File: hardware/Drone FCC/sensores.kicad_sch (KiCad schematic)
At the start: 17 parts, among them J1 Conn_02x03_Counter_Clockwise, J19 GPS M8N, J2 Conector GPS Auxiliar, J20 Conector Magnetómetro I2C DF13, U1 ICM-42688-V, U2 ILPS22QSTR

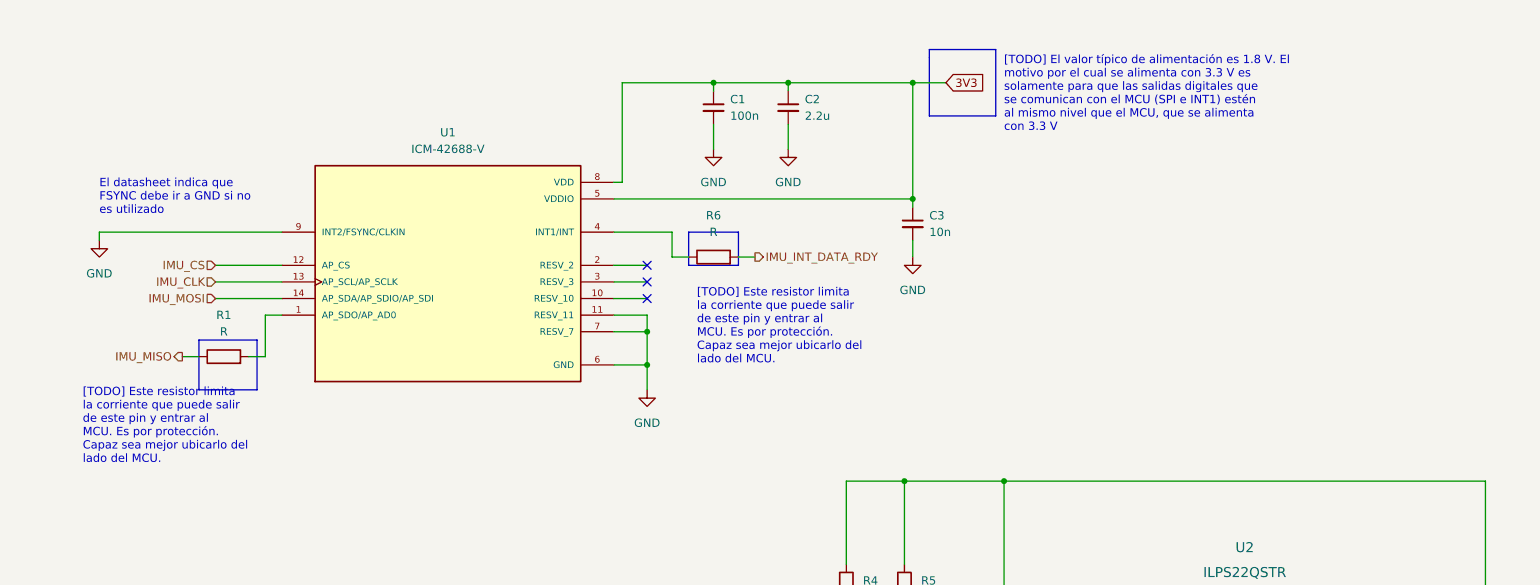
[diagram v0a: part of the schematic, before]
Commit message: finished IMU basic schematic
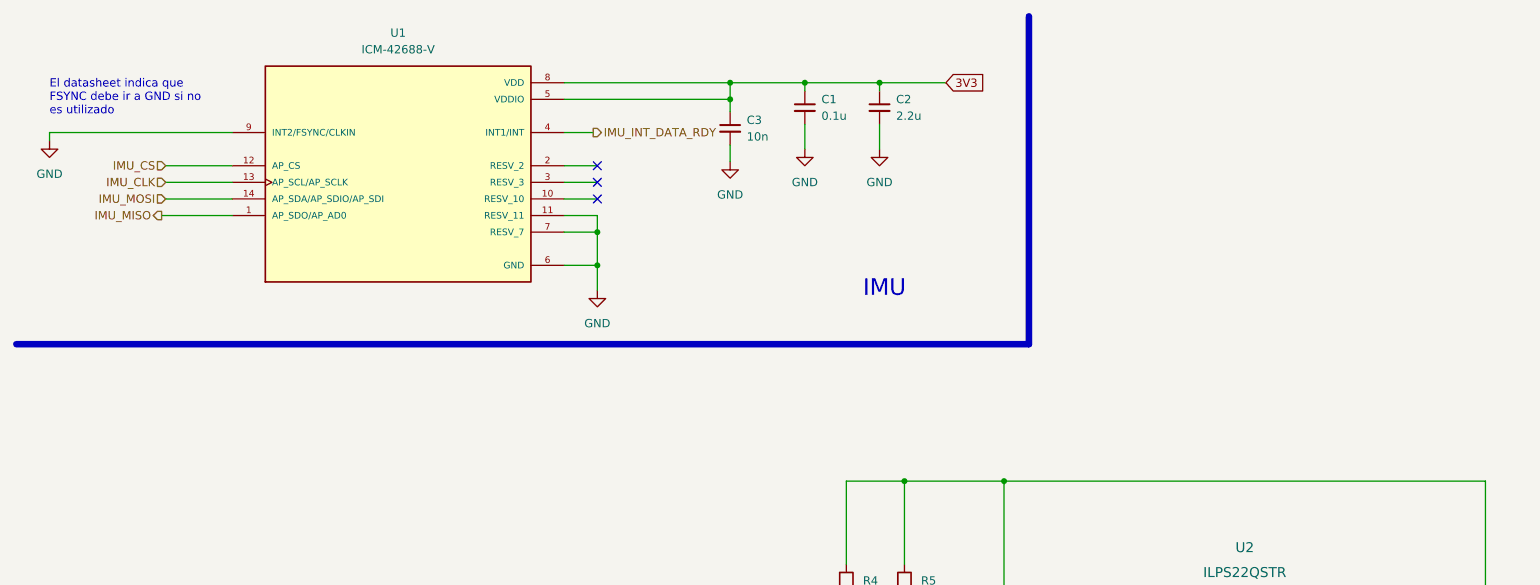
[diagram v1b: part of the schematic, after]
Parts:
- removed R1, R6: R, symbol Device:R
- C1: value 100n -> 0.1u
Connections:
- net IMU_INT_DATA_RDY: now also U1.4 (INT1/INT)
- net IMU_MISO: now also U1.1 (AP_SDO/AP_AD0)
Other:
- note added: "IMU"
- note removed: "[TODO] El valor típico de alimentación es 1.8 V. El motivo por el cual se alimenta con 3.3 V es solamente para que las salidas digitales que se comunican con el MCU (SPI e INT1) estén al mismo nivel que el MCU, que se alimenta con 3.3 V"
- note removed: "[TODO] Este resistor limita la corriente que puede salir de este pin y entrar al MCU. Es por protección. Capaz sea mejor ubicarlo del lado del MCU."
- moved on the sheet: C1, C2, C3, U1
